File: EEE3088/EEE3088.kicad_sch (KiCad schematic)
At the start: 0 parts

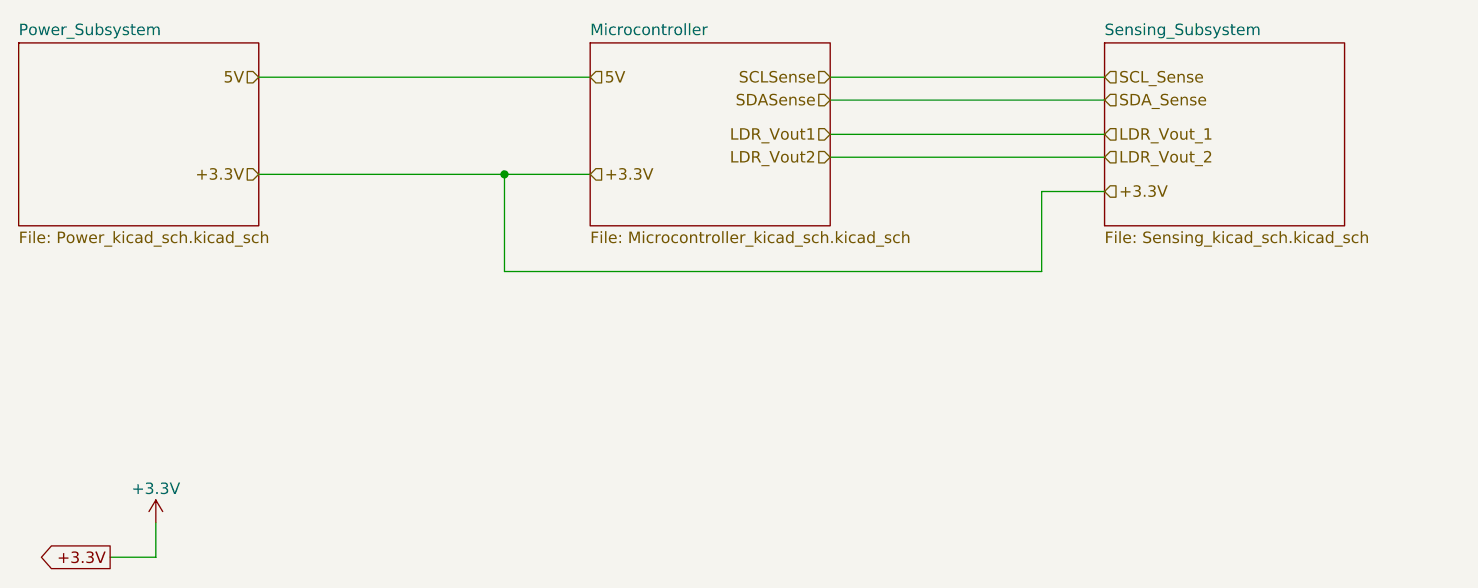
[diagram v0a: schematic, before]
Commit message: Sense_Wiring
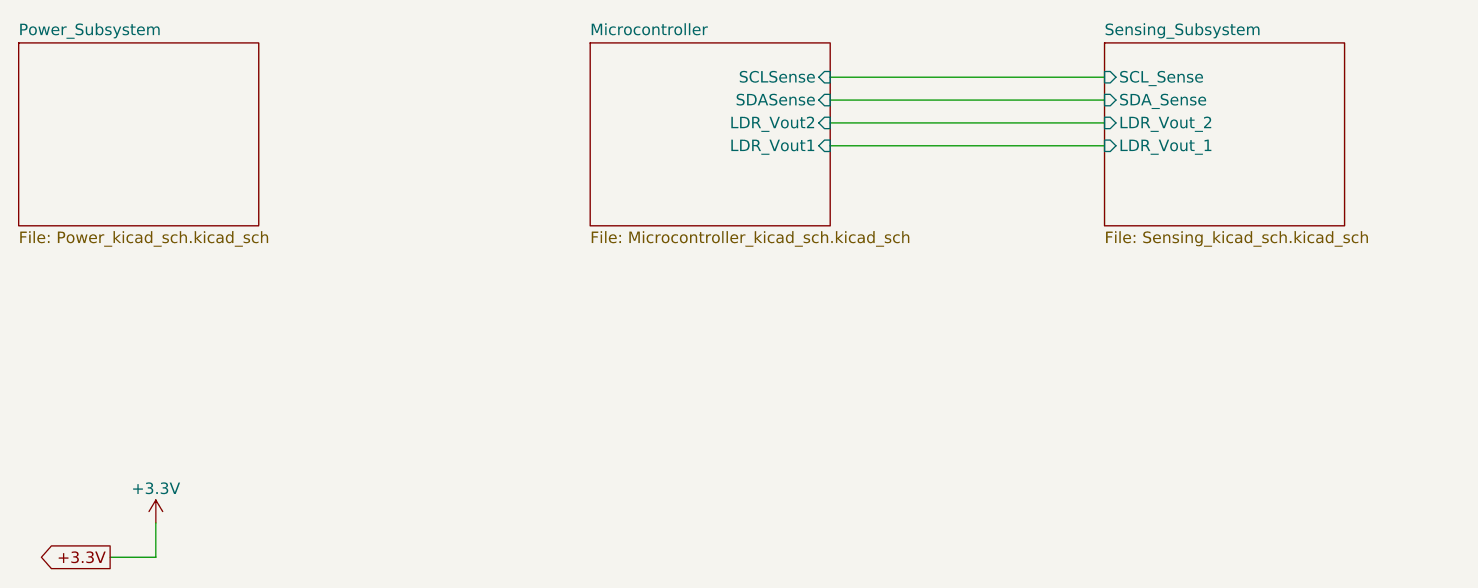
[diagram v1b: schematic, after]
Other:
- sheet Microcontroller ports: added LDR_Vout1, LDR_Vout2, SCLSense, SDASense; removed none
- sheet Sensing_Subsystem ports: added LDR_Vout_1, LDR_Vout_2, SCL_Sense, SDA_Sense; removed none
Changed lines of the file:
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@@
     (company "UCT")
   )
-  (junction (at 133.985 94.615) (diameter 0) (color 0 0 0 0)
+  (wire (pts (xy 170.18 86.36) (xy 200.66 86.36))
+    (stroke (width 0) (type default))
   )
-  (wire (pts (xy 133.985 94.615) (xy 143.51 94.615))
+  (wire (pts (xy 170.18 83.82) (xy 200.66 83.82))
     (stroke (width 0) (type default))
   )
@@
     (stroke (width 0) (type default))
   )
-  (wire (pts (xy 133.985 105.41) (xy 193.675 105.41))
+  (wire (pts (xy 170.18 91.44) (xy 200.66 91.44))
     (stroke (width 0) (type default))
   )
-  (wire (pts (xy 106.68 94.615) (xy 133.985 94.615))
-    (stroke (width 0) (type default))
-  )
-  (wire (pts (xy 170.18 92.71) (xy 200.66 92.71))
-    (stroke (width 0) (type default))
-  )
-  (wire (pts (xy 193.675 105.41) (xy 193.675 96.52))
-    (stroke (width 0) (type default))
-  )
-  (wire (pts (xy 170.18 86.36) (xy 200.66 86.36))
-    (stroke (width 0) (type default))
-  )
-  (wire (pts (xy 133.985 94.615) (xy 133.985 105.41))
-    (stroke (width 0) (type default))
-  )
-  (wire (pts (xy 170.18 83.82) (xy 200.66 83.82))
-    (stroke (width 0) (type default))
-  )
-  (wire (pts (xy 170.18 90.17) (xy 200.66 90.17))
+  (wire (pts (xy 170.18 88.9) (xy 200.66 88.9))
     (stroke (width 0) (type default))
   )
   (wire (pts (xy 95.25 133.35) (xy 95.25 137.16))
-    (stroke (width 0) (type default))
-  )
-  (wire (pts (xy 106.68 83.82) (xy 143.51 83.82))
-    (stroke (width 0) (type default))
-  )
-  (wire (pts (xy 193.675 96.52) (xy 200.66 96.52))
     (stroke (width 0) (type default))
   )
@@
       (effects (font (size 1.27 1.27)) (justify right) hide)
     )
-  )
-  (hierarchical_label "LDR_Vout_1" (shape input) (at 200.66 90.17 0) (fields_autoplaced)
-    (effects (font (size 1.27 1.27)) (justify left))
-  )
-  (hierarchical_label "+3.3V" (shape input) (at 200.66 96.52 0) (fields_autoplaced)
-    (effects (font (size 1.27 1.27)) (justify left))
-  )
-  (hierarchical_label "SCLSense" (shape input) (at 170.18 83.82 180) (fields_autoplaced)
-    (effects (font (size 1.27 1.27)) (justify right))
-  )
-  (hierarchical_label "LDR_Vout2" (shape input) (at 170.18 92.71 180) (fields_autoplaced)
-    (effects (font (size 1.27 1.27)) (justify right))
-  )
-  (hierarchical_label "+3.3V" (shape input) (at 106.68 94.615 180) (fields_autoplaced)
-    (effects (font (size 1.27 1.27)) (justify right))
-  )
-  (hierarchical_label "+3.3V" (shape input) (at 143.51 94.615 0) (fields_autoplaced)
-    (effects (font (size 1.27 1.27)) (justify left))
-  )
-  (hierarchical_label "5V" (shape input) (at 143.51 83.82 0) (fields_autoplaced)
-    (effects (font (size 1.27 1.27)) (justify left))
-  )
-  (hierarchical_label "LDR_Vout_2" (shape input) (at 200.66 92.71 0) (fields_autoplaced)
-    (effects (font (size 1.27 1.27)) (justify left))
-  )
-  (hierarchical_label "5V" (shape input) (at 106.68 83.82 180) (fields_autoplaced)
-    (effects (font (size 1.27 1.27)) (justify right))
-  )
-  (hierarchical_label "LDR_Vout1" (shape input) (at 170.18 90.17 180) (fields_autoplaced)
-    (effects (font (size 1.27 1.27)) (justify right))
-  )
-  (hierarchical_label "SDA_Sense" (shape input) (at 200.66 86.36 0) (fields_autoplaced)
-    (effects (font (size 1.27 1.27)) (justify left))
-  )
-  (hierarchical_label "SDASense" (shape input) (at 170.18 86.36 180) (fields_autoplaced)
-    (effects (font (size 1.27 1.27)) (justify right))
-  )
-  (hierarchical_label "SCL_Sense" (shape input) (at 200.66 83.82 0) (fields_autoplaced)
-    (effects (font (size 1.27 1.27)) (justify left))
   )
   (symbol (lib_id "power:+3.3V") (at 95.25 133.35 0) (unit 1)
@@
       (effects (font (size 1.27 1.27)) (justify left top))
     )
+    (pin "SCLSense" input (at 170.18 83.82 0)
+      (effects (font (size 1.27 1.27)) (justify right))
+    )
+    (pin "LDR_Vout2" input (at 170.18 88.9 0)
+      (effects (font (size 1.27 1.27)) (justify right))
+    )
+    (pin "SDASense" input (at 170.18 86.36 0)
+      (effects (font (size 1.27 1.27)) (justify right))
+    )
+    (pin "LDR_Vout1" input (at 170.18 91.44 0)
+      (effects (font (size 1.27 1.27)) (justify right))
+    )
     (instances
       (project "EEE3088"
@@
       (effects (font (size 1.27 1.27)) (justify left top))
     )
+    (pin "SCL_Sense" input (at 200.66 83.82 180)
+      (effects (font (size 1.27 1.27)) (justify left))
+    )
+    (pin "SDA_Sense" input (at 200.66 86.36 180)
+      (effects (font (size 1.27 1.27)) (justify left))
+    )
+    (pin "LDR_Vout_2" input (at 200.66 88.9 180)
+      (effects (font (size 1.27 1.27)) (justify left))
+    )
+    (pin "LDR_Vout_1" input (at 200.66 91.44 180)
+      (effects (font (size 1.27 1.27)) (justify left))
+    )
     (instances
